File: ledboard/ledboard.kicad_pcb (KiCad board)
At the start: 2 copper layers, 88.9 x 58.4 mm, 59 parts, among them J1 LEFT, J2 PWR_L, J3 RIGHT, J4 PWR_R, J5 Conn_01x03_Male, J6 Conn_01x03_Male, J7 Conn_01x02_Male, K1 FINDER-40.31, Q1 BC547, U1 AL8860, U2 AL8860, U3 LM22676MR-5, U4 RASPBERRYPI4_4GB

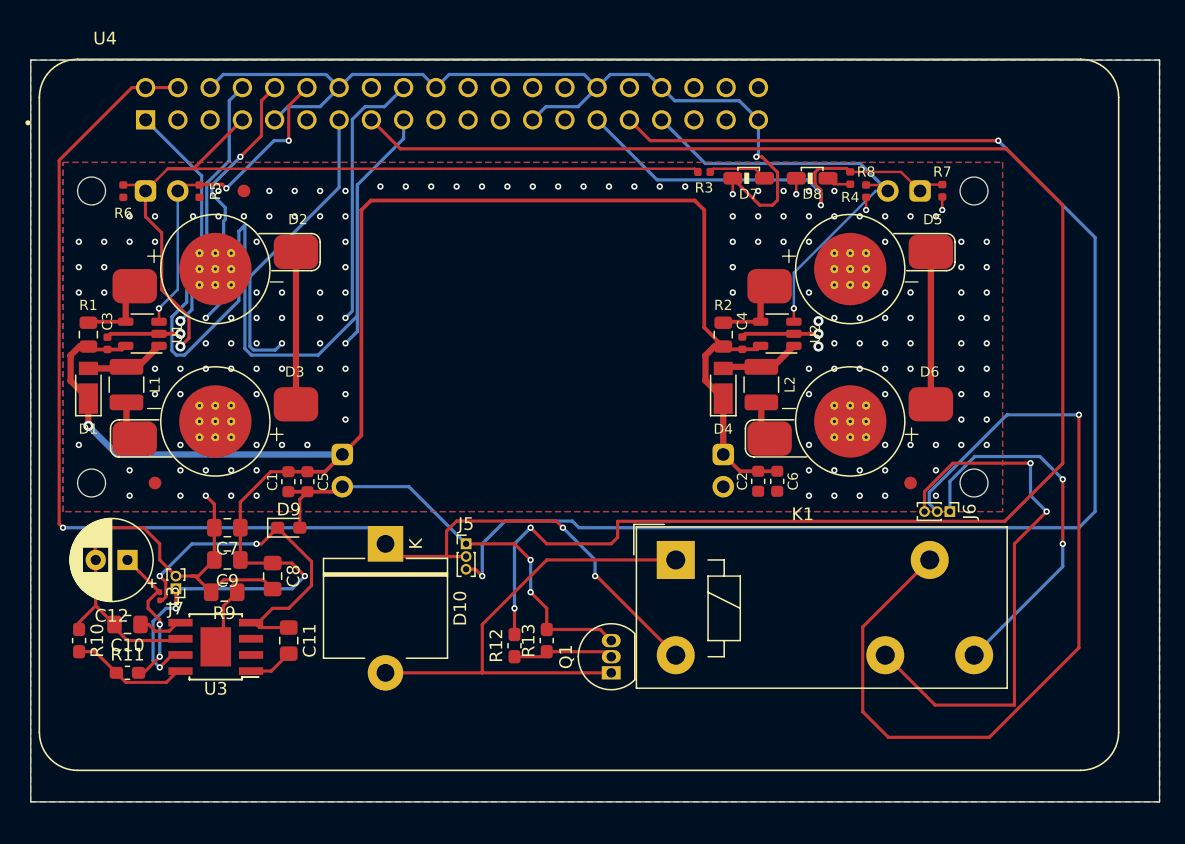
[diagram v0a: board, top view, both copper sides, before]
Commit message: last
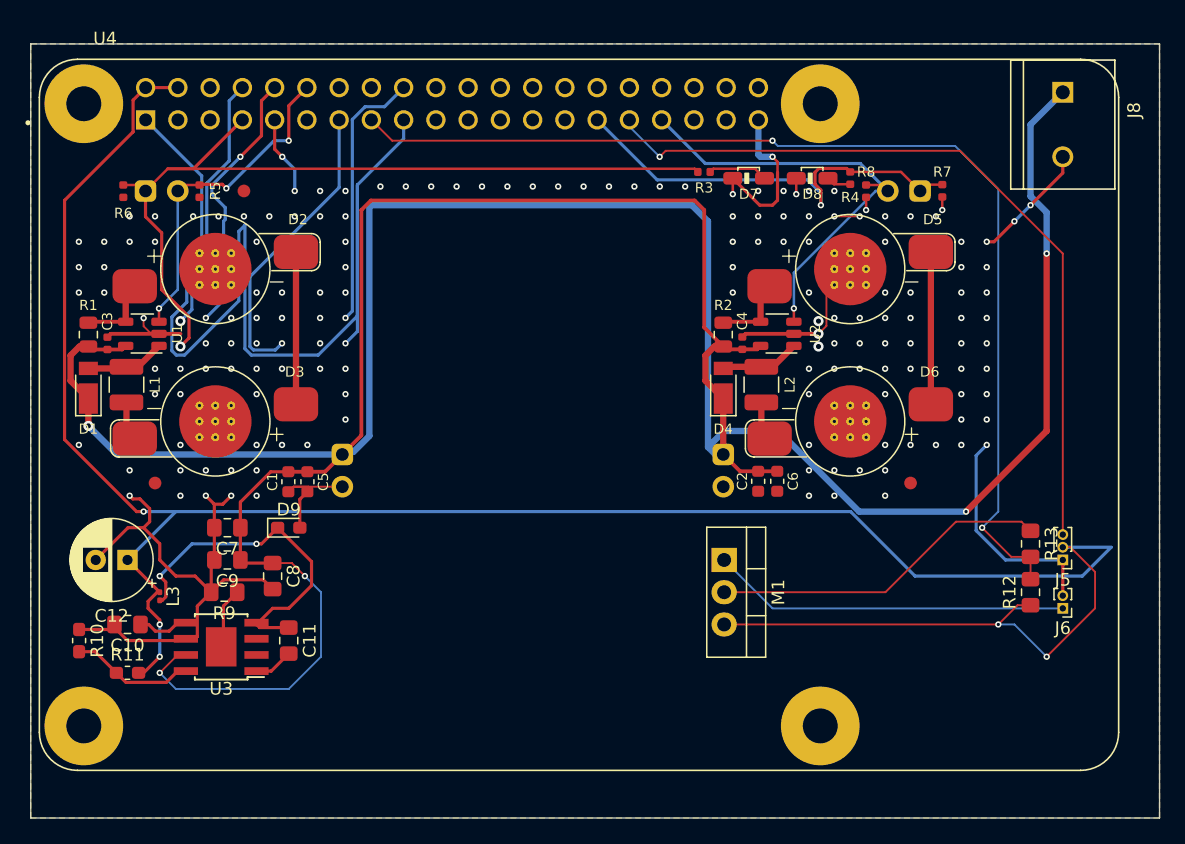
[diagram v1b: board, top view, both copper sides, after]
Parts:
- removed D10: D, Diode_THT:D_5KP_P10.16mm_Horizontal
- removed J7: Conn_01x02_Male, Connector_PinHeader_1.00mm:PinHeader_1x02_P1.00mm_Vertical
- removed K1: FINDER-40.31, Relay_THT:Relay_SPDT_Finder_40.31
- removed Q1: BC547, Package_TO_SOT_THT:TO-92_Inline
- removed the REF** at (35.2, 65.2)
- removed the REF** at (104.8, 65.2)
- removed the REF** at (35.2, 42.2)
- removed the REF** at (104.8, 42.2)
- added J8: Conn_01x02_Shielded, Connector:TE_282837-2, F.Cu at (111.7, 37.0)
- added M1: MPMOS, Package_TO_SOT_THT:TO-220-3_Vertical, F.Cu at (85.1, 71.3)
- J6: value Conn_01x03_Male -> Conn_01x02_Male; footprint Connector_PinHeader_1.00mm:PinHeader_1x03_P1.00mm_Vertical -> Connector_PinHeader_1.00mm:PinHeader_1x02_P1.00mm_Vertical
- R12: value 1k -> 10k; footprint Resistor_SMD:R_0603_1608Metric_Pad1.05x0.95mm_HandSolder -> Resistor_SMD:R_0805_2012Metric_Pad1.15x1.40mm_HandSolder
- R13: value 1k -> 150; footprint Resistor_SMD:R_0603_1608Metric_Pad1.05x0.95mm_HandSolder -> Resistor_SMD:R_0805_2012Metric_Pad1.15x1.40mm_HandSolder
- moved J5 47.0 mm to (111.7, 71.3), turned to 180 degrees
- moved R12 40.9 mm to (109.2, 73.8)
- moved R13 38.9 mm to (109.2, 70.0), turned to 270 degrees
- moved J6 11.7 mm to (111.7, 75.1), turned to 180 degrees
- moved U3 0.43 mm to (45.5, 78.2)
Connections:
- C1 pad 2: 0 -> GND
- C10 pad 2: 0 -> GND
- C12 pad 1: Net-(C12-Pad1) -> +5V
- C12 pad 2: 0 -> GND
- C2 pad 2: 0 -> GND
- C3 pad 2: 0 -> GND
- C4 pad 2: 0 -> GND
- C5 pad 2: 0 -> GND
- C6 pad 2: 0 -> GND
- C7 pad 2: 0 -> GND
- C8 pad 2: 0 -> GND
- C9 pad 2: 0 -> GND
- D2 pad 3: 0 -> GND
- D3 pad 3: 0 -> GND
- D5 pad 3: 0 -> GND
- D6 pad 3: 0 -> GND
- D7 pad 1: 0 -> GND
- D8 pad 1: 0 -> GND
- D9 pad 2: 0 -> GND
- J2 pad 2: 0 -> GND
- J4 pad 2: 0 -> GND
- J5 pad 1: 0 -> GND
- J6 pad 2: Net-(J6-Pad2) -> GND
- L3 pad 1: Net-(C12-Pad1) -> +5V
- R10 pad 1: 0 -> GND
- R11 pad 2: Net-(C12-Pad1) -> +5V
- R12 pad 1: Net-(Q1-Pad2) -> +5V
- R13 pad 1: Net-(Q1-Pad2) -> Net-(M1-Pad2)
- R13 pad 2: 0 -> /FAN_PIN
- R5 pad 2: 0 -> GND
- R6 pad 2: 0 -> GND
- R7 pad 2: 0 -> GND
- R8 pad 2: 0 -> GND
- R9 pad 2: 0 -> GND
- U1 pad 2: 0 -> GND
- U2 pad 2: 0 -> GND
- U3 pad 2: Net-(U3-Pad2) -> (no net)
- U3 pad 3: Net-(U3-Pad3) -> (no net)
- U3 pad 6: 0 -> GND
- U4 pad 10: Net-(U4-Pad10) -> (no net)
- U4 pad 11: Net-(U4-Pad11) -> (no net)
- U4 pad 13: Net-(U4-Pad13) -> (no net)
- U4 pad 14: 0 -> GND
- U4 pad 16: Net-(U4-Pad16) -> (no net)
- U4 pad 18: Net-(U4-Pad18) -> (no net)
- U4 pad 19: Net-(U4-Pad19) -> (no net)
- U4 pad 20: 0 -> GND
- U4 pad 21: Net-(U4-Pad21) -> (no net)
- U4 pad 22: Net-(U4-Pad22) -> (no net)
- U4 pad 23: Net-(U4-Pad23) -> (no net)
- U4 pad 24: Net-(U4-Pad24) -> (no net)
- U4 pad 25: 0 -> GND
- U4 pad 26: Net-(U4-Pad26) -> (no net)
- U4 pad 27: Net-(U4-Pad27) -> (no net)
- U4 pad 28: Net-(U4-Pad28) -> (no net)
- U4 pad 3: Net-(U4-Pad3) -> (no net)
- U4 pad 30: 0 -> GND
- U4 pad 32: Net-(U4-Pad32) -> (no net)
- U4 pad 34: 0 -> GND
- U4 pad 35: Net-(U4-Pad35) -> (no net)
- U4 pad 36: Net-(U4-Pad36) -> (no net)
- U4 pad 37: Net-(U4-Pad37) -> (no net)
- U4 pad 38: Net-(U4-Pad38) -> (no net)
- U4 pad 40: Net-(U4-Pad40) -> (no net)
- U4 pad 5: Net-(U4-Pad5) -> (no net)
- U4 pad 6: 0 -> GND
- U4 pad 8: Net-(U4-Pad8) -> (no net)
- U4 pad 9: 0 -> GND
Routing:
- net 0: track 166.5 -> 0.00 mm, vias 159 -> 0
- net +12V: track 148.8 -> 280.0 mm, vias 4 -> 5
- net GND: track 0.00 -> 126.3 mm, vias 0 -> 155
- net (no net): track 0.00 -> 86.6 mm, vias 0 -> 5
- net +5V: track 99.0 -> 182.9 mm, vias 3 -> 5
- net Net-(J6-Pad2): track 69.3 -> 0.00 mm, vias 1 -> 0
- net /PWM_LED: track 115.9 -> 61.3 mm, vias 2 -> 1
- net /FAN_PIN: track 132.3 -> 85.3 mm
- net Net-(J6-Pad3): track 43.3 -> 0.00 mm, vias 2 -> 0
- net Net-(D10-Pad2): track 38.9 -> 0.00 mm
- net Net-(M1-Pad2): track 0.00 -> 26.7 mm
- net Net-(U4-Pad13): track 23.6 -> 0.00 mm, vias 1 -> 0
- net Net-(U4-Pad10): track 21.3 -> 0.00 mm, vias 2 -> 0
- net Net-(U4-Pad18): track 20.9 -> 0.00 mm, vias 1 -> 0
- net Net-(U4-Pad8): track 20.8 -> 0.00 mm, vias 1 -> 0
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- added copper zone on B.Cu, net GND
- added copper zone on F.Cu, net GND
- removed copper zone on B.Cu, net 0
- removed copper zone on F.Cu, net 0
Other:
- board size 88.9 x 58.4 mm -> 88.9 x 61 mm

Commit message: hole
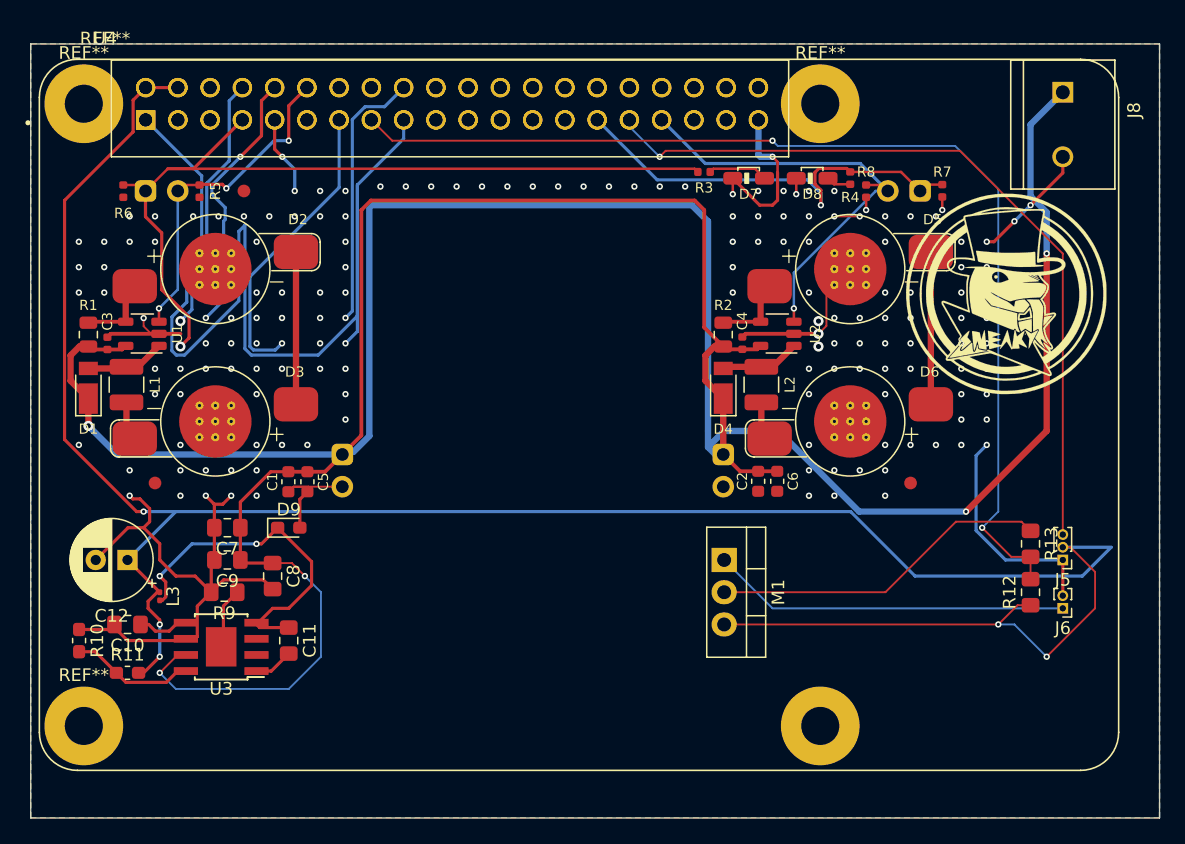
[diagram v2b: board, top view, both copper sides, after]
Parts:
- added ?: MountingHole_3mm_Pad, MountingHole:MountingHole_3mm_Pad, F.Cu at (92.6, 84.4)
- added G***: LOGO, KiCad raspberry pi:LOGO, F.Cu at (107.3, 50.4)
- added REF**: MODULE_RASPBERRYPI4_4GB, KiCad raspberry pi:MODULE_RASPBERRYPI4_4GB_HOLE, F.Cu at (73.6, 59.9)
- added REF**: MountingHole_3mm_Pad, MountingHole:MountingHole_3mm_Pad, F.Cu at (34.6, 84.4)
- added REF**: MountingHole_3mm_Pad, MountingHole:MountingHole_3mm_Pad, F.Cu at (92.6, 35.4)
- added REF**: MountingHole_3mm_Pad, MountingHole:MountingHole_3mm_Pad, F.Cu at (34.6, 35.4)
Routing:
- net (no net): track 86.6 -> 177.0 mm, vias 5 -> 8
- net Net-(U4-Pad1): track 84.2 -> 0.00 mm, vias 1 -> 0
- net GND: track 126.3 -> 120.0 mm, vias 155 -> 153

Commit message: wire
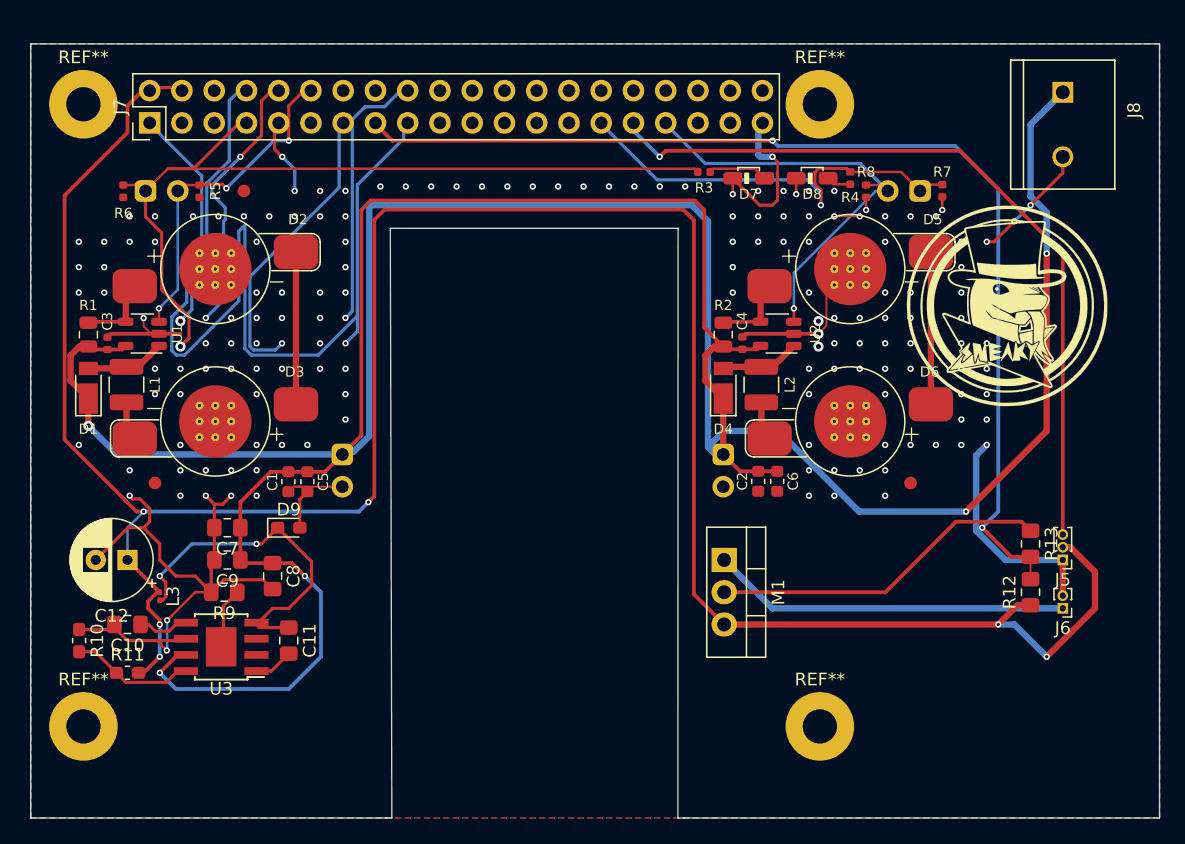
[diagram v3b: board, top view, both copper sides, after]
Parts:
- removed ?: MountingHole_3mm_Pad, MountingHole:MountingHole_3mm_Pad
- removed the REF** at (73.6, 59.9)
- removed the REF** at (34.6, 84.4)
- removed the REF** at (92.6, 35.4)
- removed the REF** at (34.6, 35.4)
- removed U4: RASPBERRYPI4_4GB, KiCad raspberry pi:MODULE_RASPBERRYPI4_4GB
- added J7: Conn_02x20_Odd_Even, Connector_PinHeader_2.54mm:PinHeader_2x20_P2.54mm_Vertical, F.Cu at (39.8, 36.9)
- added REF**: MountingHole_2.7mm_Pad, MountingHole:MountingHole_2.7mm_Pad, F.Cu at (34.6, 84.4)
- added REF**: MountingHole_2.7mm_Pad, MountingHole:MountingHole_2.7mm_Pad, F.Cu at (92.6, 84.4)
- added REF**: MountingHole_2.7mm_Pad, MountingHole:MountingHole_2.7mm_Pad, F.Cu at (92.6, 35.4)
- added REF**: MountingHole_2.7mm_Pad, MountingHole:MountingHole_2.7mm_Pad, F.Cu at (34.6, 35.4)
- moved G*** 0.95 mm to (107.4, 51.3)
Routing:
- net +5V: track 182.9 -> 197.9 mm, vias 5 -> 6
- net GND: track 120.0 -> 123.2 mm, vias 153 -> 152
- net Net-(J7-Pad28): vias 0 -> 1
- net Net-(J7-Pad27): vias 0 -> 1
- net (no net): vias 8 -> 9
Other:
- outline, holes or cut-outs redrawn
